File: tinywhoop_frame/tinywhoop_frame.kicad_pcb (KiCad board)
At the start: 2 copper layers, 90 x 90 mm, 18 parts, among them J1 ESP_conn1, J2 ESP_conn2, J3 ESP_Unused_Pins1, J5 Batt_conn, J6 Conn_02x03_Counter_Clockwise, Q1 2N7002, Q2 2N7002, Q3 2N7002, Q4 2N7002

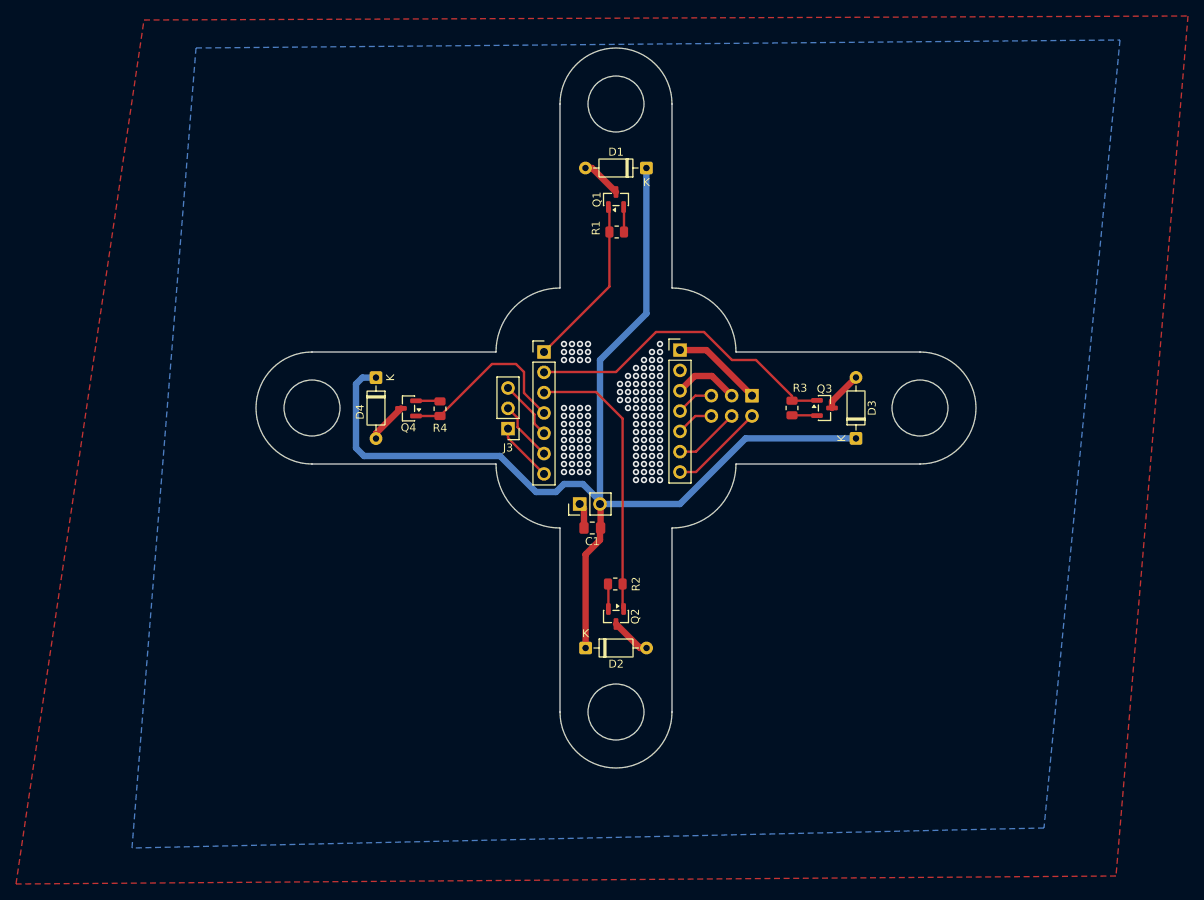
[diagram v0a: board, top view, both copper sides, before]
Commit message: updated pcb
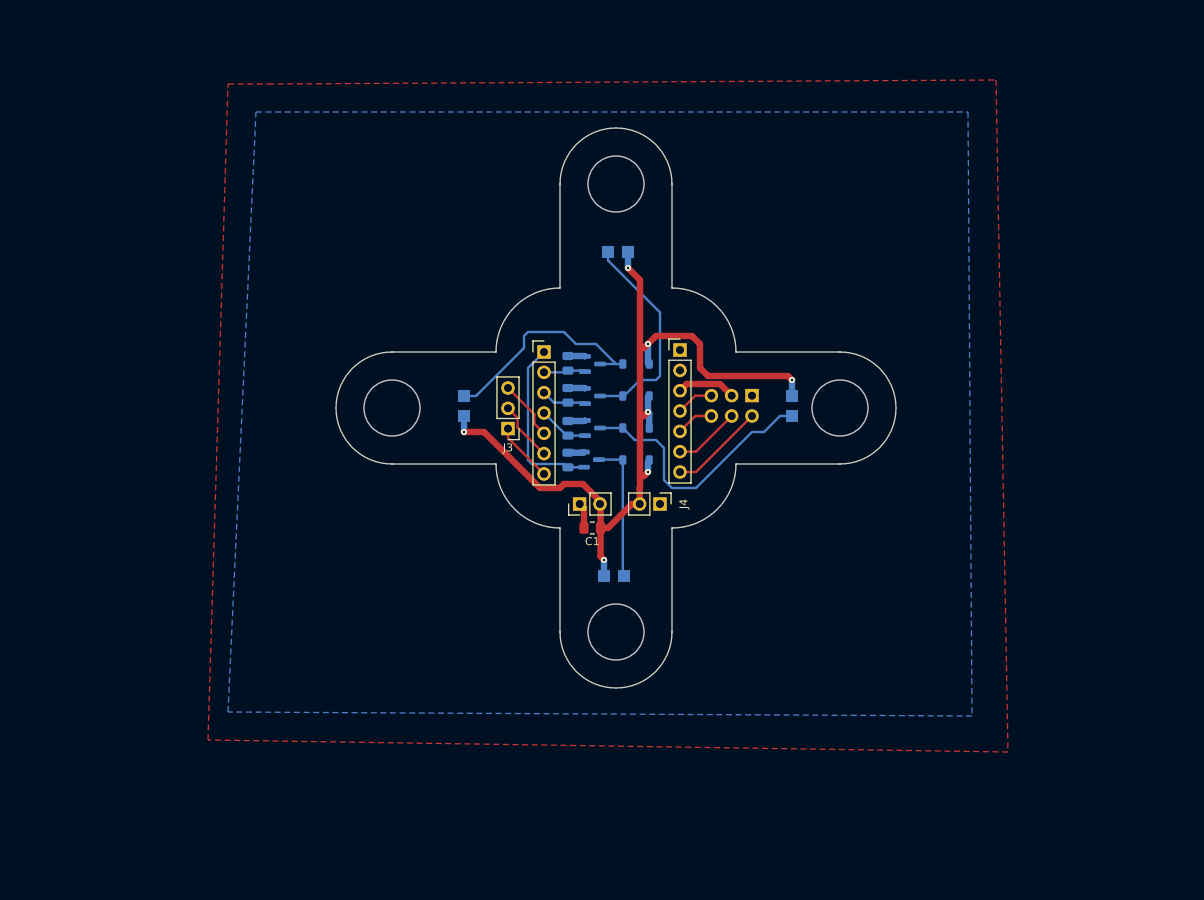
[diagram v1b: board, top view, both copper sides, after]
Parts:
- added J4: Batt_conn_MCU, Connector_PinHeader_2.54mm:PinHeader_1x02_P2.54mm_Vertical, F.Cu at (150.5, 79.0)
- added TP1: TestPoint, TestPoint:TestPoint_Pad_1.5x1.5mm, B.Cu at (146.0, 88.0)
- added TP2: TestPoint, TestPoint:TestPoint_Pad_1.5x1.5mm, B.Cu at (143.5, 88.0)
- added TP3: TestPoint, TestPoint:TestPoint_Pad_1.5x1.5mm, B.Cu at (144.0, 47.5)
- added TP4: TestPoint, TestPoint:TestPoint_Pad_1.5x1.5mm, B.Cu at (146.5, 47.5)
- added TP5: TestPoint, TestPoint:TestPoint_Pad_1.5x1.5mm, B.Cu at (126.0, 65.5)
- added TP6: TestPoint, TestPoint:TestPoint_Pad_1.5x1.5mm, B.Cu at (167.0, 65.5)
- added TP7: TestPoint, TestPoint:TestPoint_Pad_1.5x1.5mm, B.Cu at (167.0, 68.0)
- added TP8: TestPoint, TestPoint:TestPoint_Pad_1.5x1.5mm, B.Cu at (126.0, 68.0)
- D1, D2, D3, D4: value D -> 1N4148W; footprint Diode_THT:D_DO-35_SOD27_P7.62mm_Horizontal -> Diode_SMD:D_SOD-123; moved to B.Cu
- J5: value Batt_conn -> Batt_conn_LIPO
- Q1, Q2, Q3, Q4, R1, R2, R3, R4: moved to B.Cu
- moved D2 36.1 mm to (147.5, 61.5), turned to 180 degrees
- moved Q1 32.7 mm to (141.9, 73.5), turned to 0 degrees
- moved D4 32.6 mm to (147.5, 65.5), turned to 180 degrees
- moved D1 32.5 mm to (147.5, 69.5)
- moved Q3 29.5 mm to (142.1, 61.5)
- moved R1 29.1 mm to (139.0, 73.5), turned to 90 degrees
- moved R3 28.6 mm to (139.0, 61.4), turned to 90 degrees
- moved Q2 27.7 mm to (142.1, 65.5), turned to 0 degrees
- moved D3 27.6 mm to (147.5, 73.5), turned to 180 degrees
- moved R2 24.3 mm to (139.0, 65.4), turned to 90 degrees
- moved Q4 23.1 mm to (142.1, 69.5), turned to 0 degrees
- moved R4 16.2 mm to (139.0, 69.5)
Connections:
- D1 pad 2: Net-(D1-A) -> /M4-
- D2 pad 2: Net-(D2-A) -> /M3-
- D3 pad 2: Net-(D3-A) -> /M1-
- D4 pad 2: Net-(D4-A) -> /M2-
- J2 pad 1: /5V -> unconnected-(J2-Pin_1-Pad1)
- J6 pad 1: /5V -> unconnected-(J6-Pin_1-Pad1)
- Q1 pad 3: Net-(D1-A) -> /M1-
- Q2 pad 3: Net-(D2-A) -> /M2-
- Q3 pad 3: Net-(D3-A) -> /M3-
- Q4 pad 3: Net-(D4-A) -> /M4-
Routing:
- net BATT+: track 143.9 -> 107.7 mm, vias 0 -> 7
- net PWM2: track 40.1 -> 5.50 mm
- net /M4-: track 0.00 -> 33.2 mm
- net PWM3: track 35.3 -> 5.81 mm
- net /M3-: track 0.00 -> 27.7 mm
- net /M2-: track 0.00 -> 26.7 mm
- net /M1-: track 0.00 -> 17.6 mm
- net PWM4: track 22.8 -> 6.30 mm
- net /5V: track 11.4 -> 0.00 mm
- net Net-(D4-A): track 5.06 -> 0.00 mm
- net Net-(D3-A): track 5.06 -> 0.00 mm
- net Net-(D2-A): track 5.06 -> 0.00 mm
- net Net-(D1-A): track 5.06 -> 0.00 mm
- net BATT-: track 15.7 -> 11.7 mm, vias 122 -> 0
- net /3V3: track 8.24 -> 7.41 mm
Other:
- board size 90 x 90 mm -> 70 x 70 mm
